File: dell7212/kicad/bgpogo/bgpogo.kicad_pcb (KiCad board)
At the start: 2 copper layers, 76.7 x 72.2 mm, 10 parts, among them J1 Conn_02x13_Odd_Even, J2 USB1135-15-9-L-B_REVA1, J3 Conn_01x13, J4 PJ-019, J5 Conn_01x03, J6 Conn_01x13, J7 Conn_01x09, U1 AZ1117-5.0

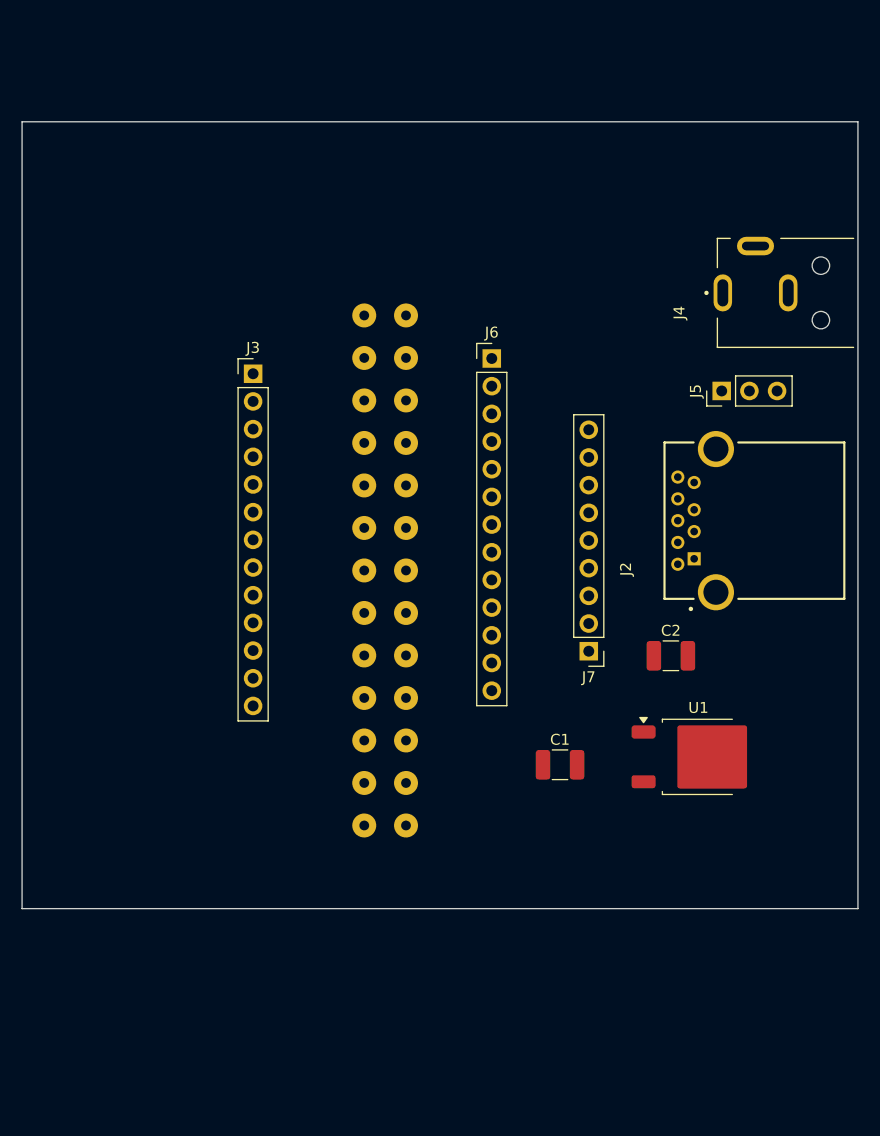
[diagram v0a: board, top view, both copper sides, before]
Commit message: board v.9
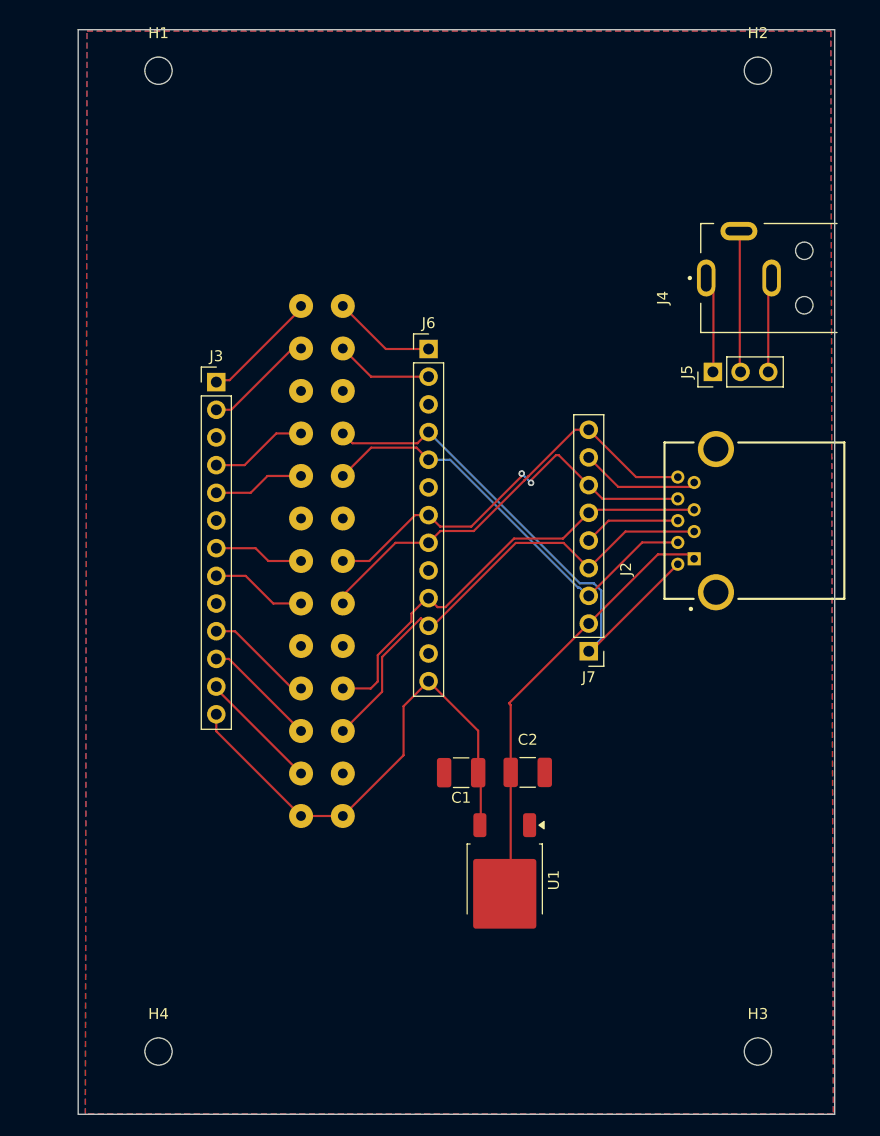
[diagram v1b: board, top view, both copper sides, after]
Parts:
- added H1: MountingHole, MountingHole:MountingHole_2.5mm, F.Cu at (81.9, 34.0)
- added H2: MountingHole, MountingHole:MountingHole_2.5mm, F.Cu at (136.9, 34.0)
- added H3: MountingHole, MountingHole:MountingHole_2.5mm, F.Cu at (136.9, 124.0)
- added H4: MountingHole, MountingHole:MountingHole_2.5mm, F.Cu at (81.9, 124.0)
- moved U1 21.1 mm to (113.7, 108.3), turned to -90 degrees
- moved C2 16.9 mm to (115.8, 98.4)
- moved C1 9.10 mm to (109.7, 98.4), turned to 180 degrees
- moved J6 5.86 mm to (106.7, 59.5)
- moved J1 5.86 mm to (92.9, 55.6)
- moved J3 3.46 mm to (87.2, 62.6)
- moved J4 2.05 mm to (138.9, 53.0)
- moved J5 1.93 mm to (132.8, 61.7)
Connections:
- J7 pad 1: +5V -> /55
- J7 pad 2: /54 -> +5V
- J7 pad 3: /53 -> /56
- J7 pad 4: GND -> /54
- J7 pad 6: /59 -> /53
- J7 pad 8: /56 -> GND
- J7 pad 9: /55 -> /59
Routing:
- net /55: track 0.00 -> 48.1 mm
- net +8V: track 0.00 -> 47.2 mm
- net /54: track 0.00 -> 44.6 mm
- net /53: track 0.00 -> 41.6 mm
- net +5V: track 0.00 -> 40.6 mm
- net /59: track 0.00 -> 39.6 mm
- net /56: track 0.00 -> 39.5 mm
- net /58: track 0.00 -> 38.4 mm, vias 0 -> 2
- net GND: track 0.00 -> 20.1 mm
- net Net-(J5-Pin_2): track 0.00 -> 13.0 mm
- net +3.3V: track 0.00 -> 11.2 mm
- net /p1: track 0.00 -> 11.2 mm
- net /p21: track 0.00 -> 10.5 mm
- net /p3: track 0.00 -> 10.1 mm
- net /p19: track 0.00 -> 9.95 mm
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- added copper zone on B.Cu, net GND
- added copper zone on F.Cu, net GND
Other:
- board size 76.7 x 72.2 mm -> 69.4 x 99.5 mm
